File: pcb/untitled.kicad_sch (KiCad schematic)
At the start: 49 parts, among them IC10 AD844_OPAMP_MEL, IC3 FOD814_OPTO_NOSHD, IC5 FOD814_OPTO_MEL, IC6 AD844_OPAMP_AL, IC7 FOD814_OPTO_AL, IC8 AD844_OPAMP_NOSHD, J4 Conn_01x02, U2 REF192_NOSHD, U3 REF192_AL, U4 REF192_MEL

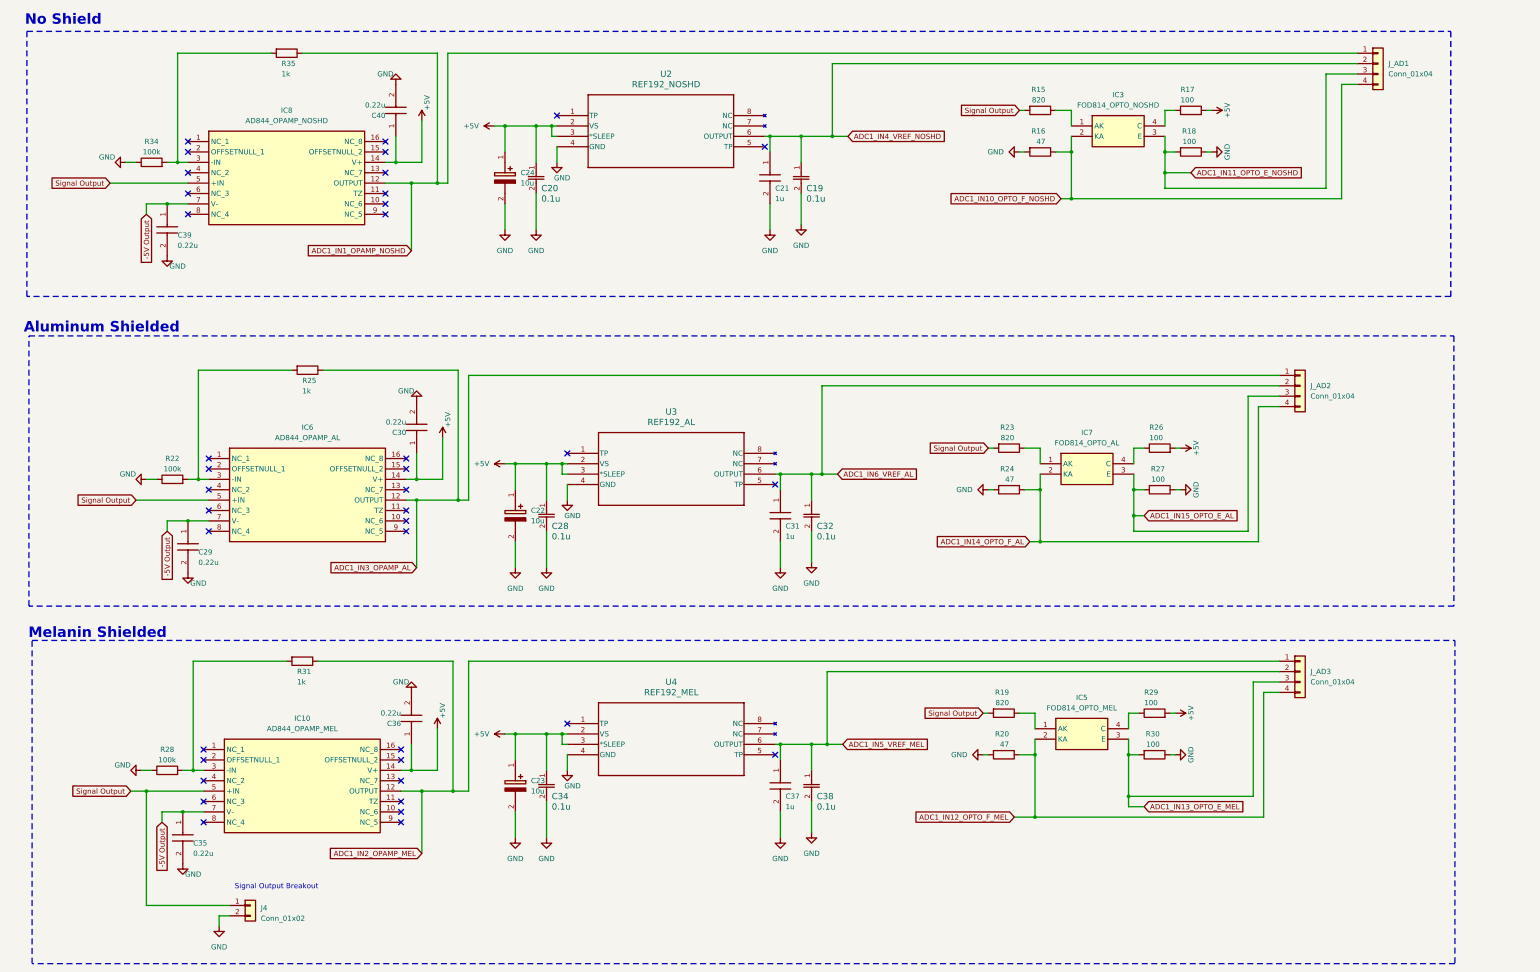
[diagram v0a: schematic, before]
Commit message: Added non-inverting amplifier
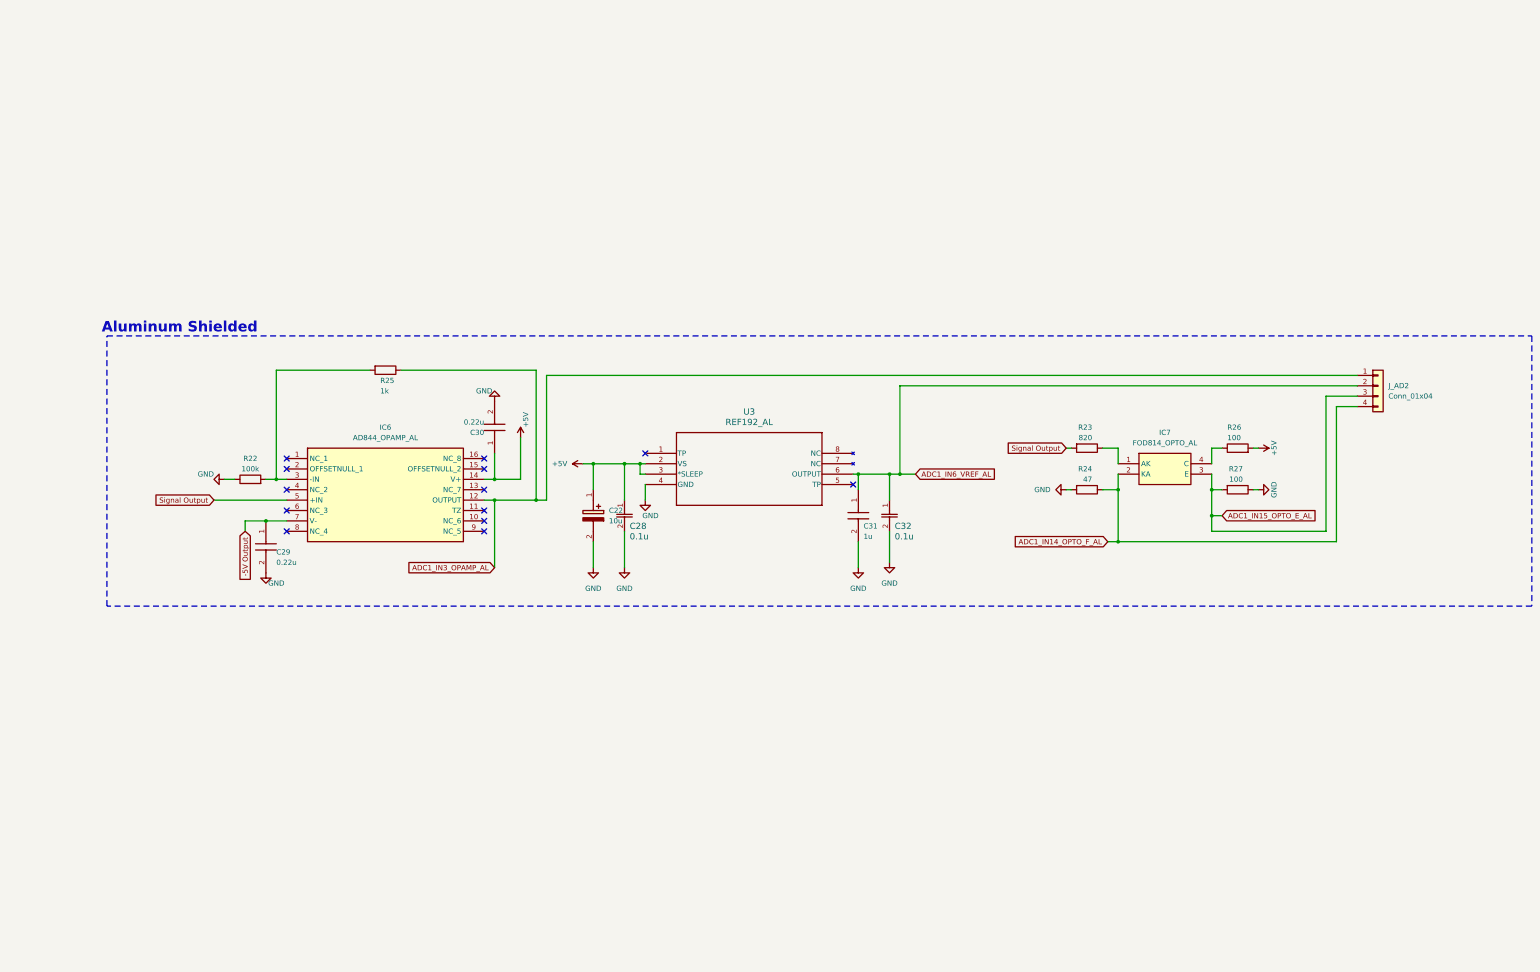
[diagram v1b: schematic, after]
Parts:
- removed C19, C20, C34, C38: 0.1u, capstone:CAPC220145_88N_KEM-0.1u, symbol capstone:C0805C104K5RAC7210
- removed C21, C37: 1u, capstone:C0805-1u, symbol capstone:C0805C105Z5VACTU-1u
- removed C23, C24: 10u, capstone:T495D, symbol capstone:T495D106K035ATE300
- removed C35, C36, C39, C40: 0.22u, capstone:C0805-0.22u, symbol capstone:C0805C224M5VACTU-0.22u
- removed IC10: AD844_OPAMP_MEL, capstone:SOIC127P1032X265-16N-AD844, symbol capstone:AD844JRZ-16-REEL7
- removed IC3: FOD814_OPTO_NOSHD, capstone:SOP254P1016X385-4N-FOD, symbol capstone:FOD814SD
- removed IC5: FOD814_OPTO_MEL, capstone:SOP254P1016X385-4N-FOD, symbol capstone:FOD814SD
- removed IC8: AD844_OPAMP_NOSHD, capstone:SOIC127P1032X265-16N-AD844, symbol capstone:AD844JRZ-16-REEL7
- removed J4: Conn_01x02, Connector_PinHeader_2.54mm:PinHeader_1x02_P2.54mm_Vertical, symbol Connector_Generic:Conn_01x02
- removed J_AD1, J_AD3: Conn_01x04, Connector_PinHeader_2.54mm:PinHeader_1x04_P2.54mm_Vertical, symbol Connector_Generic:Conn_01x04
- removed R15, R19: 820, Resistor_SMD:R_0402_1005Metric, symbol Device:R
- removed R16, R20: 47, Resistor_SMD:R_0402_1005Metric, symbol Device:R
- removed R17, R18, R29, R30: 100, Resistor_SMD:R_0402_1005Metric, symbol Device:R
- removed R28, R34: 100k, Resistor_SMD:R_0402_1005Metric, symbol Device:R
- removed R31, R35: 1k, Resistor_SMD:R_0402_1005Metric, symbol Device:R
- removed U2: REF192_NOSHD, capstone:R_8_ADI-REF, symbol capstone:REF192GSZ
- removed U4: REF192_MEL, capstone:R_8_ADI-REF, symbol capstone:REF192GSZ
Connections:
- no-connect marks 39 -> 13
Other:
- note removed: "Melanin Shielded"
- note removed: "No Shield"
- note removed: "Signal Output Breakout"
- moved on the sheet: C22, C28, C29, C30, C31, C32, IC6, IC7, J_AD2, R22, R23, R24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
